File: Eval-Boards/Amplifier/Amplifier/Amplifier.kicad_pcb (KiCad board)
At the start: 2 copper layers, 8 parts

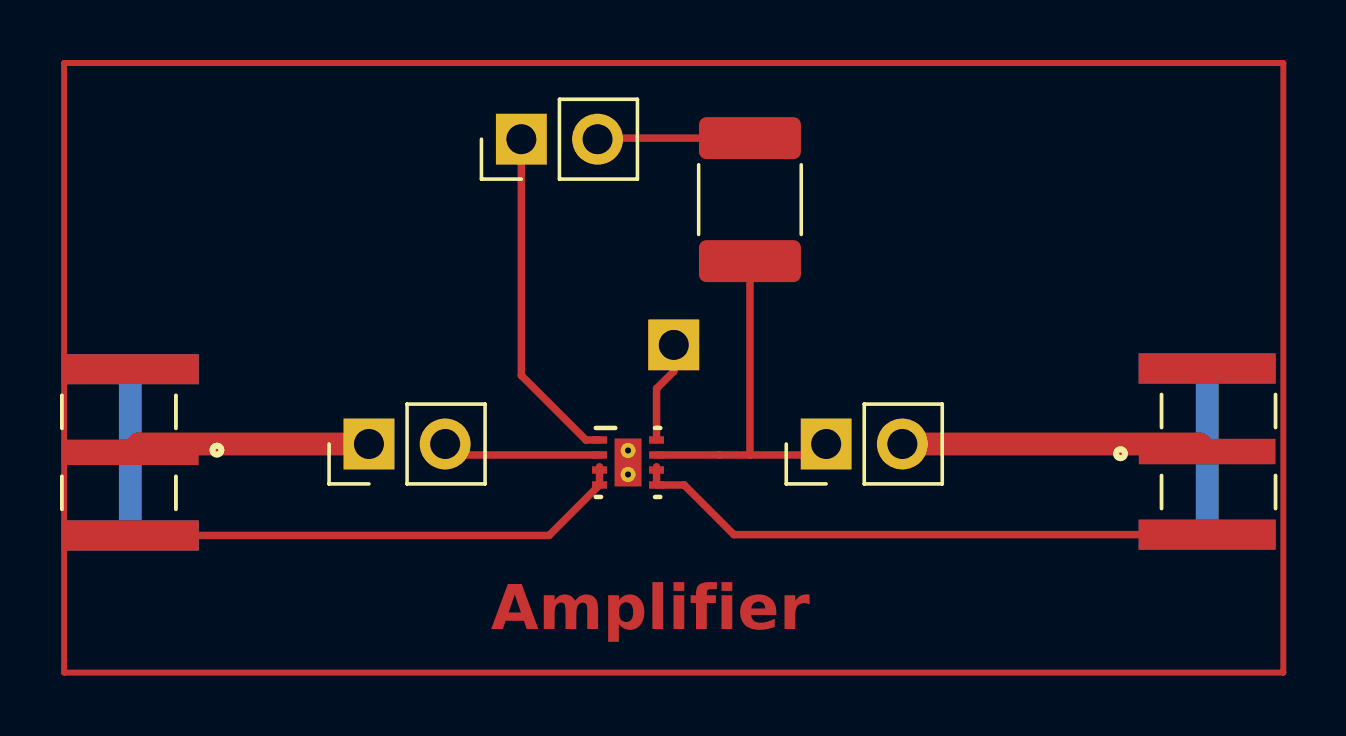
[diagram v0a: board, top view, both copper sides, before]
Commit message: Alot of stuff. Eval board for amp and VCO test
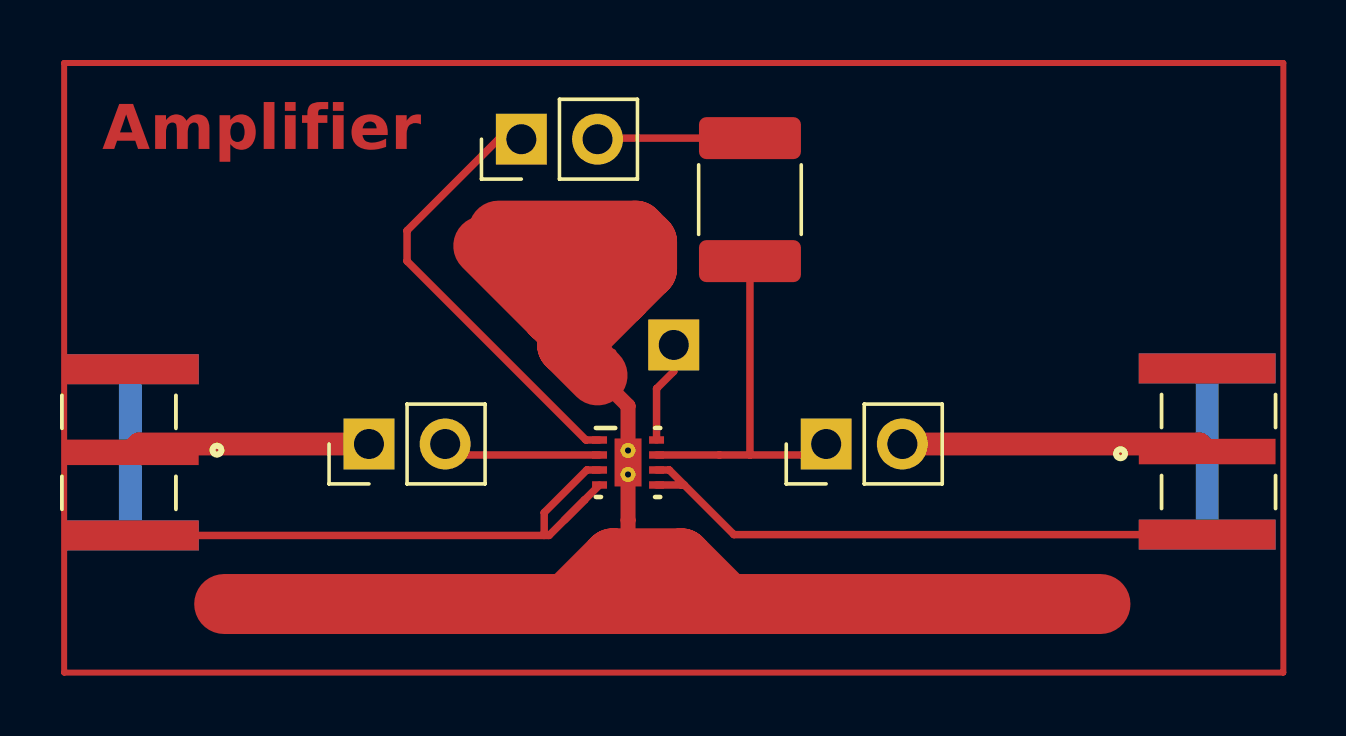
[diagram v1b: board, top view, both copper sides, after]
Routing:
- net (no net): track 103.5 -> 179.9 mm
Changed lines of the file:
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@@
   (gr_rect (start 40.64 35.56) (end 81.28 55.88)
     (stroke (width 0.2) (type default)) (fill none) (layer "F.Cu"))
-  (gr_text "Amplifier" (at 54.864 54.61) (layer "F.Cu")
+  (gr_text "Amplifier" (at 41.91 38.608) (layer "F.Cu")
     (effects (font (size 1.5 1.5) (thickness 0.3) bold) (justify left bottom))
   )
   (segment (start 63.5 48.625999) (end 65.674001 48.625999) (width 0.25) (layer "F.Cu") (net 0))
   (segment (start 53.705999 48.625999) (end 53.34 48.26) (width 0.25) (layer "F.Cu") (net 0))
+  (segment (start 75.184 53.594) (end 57.404 53.594) (width 2) (layer "F.Cu") (net 0))
   (segment (start 43.123001 48.26) (end 42.845001 48.538) (width 0.762) (layer "F.Cu") (net 0))
+  (segment (start 60.810001 49.126001) (end 61.309999 49.625999) (width 0.25) (layer "F.Cu") (net 0))
+  (segment (start 57.311998 50.8) (end 57.992999 50.118999) (width 0.25) (layer "F.Cu") (net 0))
+  (segment (start 61.214 49.625999) (end 61.309999 49.625999) (width 0.25) (layer "F.Cu") (net 0))
+  (segment (start 54.61 41.656) (end 56.896 43.942) (width 2) (layer "F.Cu") (net 0))
+  (segment (start 60.386001 49.625999) (end 61.214 49.625999) (width 0.25) (layer "F.Cu") (net 0))
+  (segment (start 61.214 53.594) (end 61.468 53.594) (width 0.25) (layer "F.Cu") (net 0))
+  (segment (start 58.485999 48.126) (end 58.032 48.126) (width 0.25) (layer "F.Cu") (net 0))
   (segment (start 50.8 48.26) (end 43.123001 48.26) (width 0.762) (layer "F.Cu") (net 0))
-  (segment (start 60.386001 49.625999) (end 61.309999 49.625999) (width 0.25) (layer "F.Cu") (net 0))
+  (segment (start 60.386001 49.126001) (end 60.810001 49.126001) (width 0.25) (layer "F.Cu") (net 0))
+  (segment (start 57.404 44.45) (end 57.404 44.958) (width 2) (layer "F.Cu") (net 0))
+  (segment (start 58.42 45.974) (end 58.166 45.72) (width 0.25) (layer "F.Cu") (net 0))
+  (segment (start 58.485999 49.126001) (end 58.061999 49.126001) (width 0.25) (layer "F.Cu") (net 0))
+  (segment (start 58.039 44.45) (end 57.404 44.45) (width 2) (layer "F.Cu") (net 0))
   (segment (start 60.386001 48.625999) (end 62.484 48.625999) (width 0.25) (layer "F.Cu") (net 0))
+  (segment (start 58.928 46.482) (end 58.928 45.212) (width 0.25) (layer "F.Cu") (net 0))
+  (segment (start 58.032 48.126) (end 52.07 42.164) (width 0.25) (layer "F.Cu") (net 0))
+  (segment (start 57.404 53.594) (end 58.928 52.07) (width 2) (layer "F.Cu") (net 0))
   (segment (start 60.386001 46.416001) (end 60.96 45.842002) (width 0.25) (layer "F.Cu") (net 0))
   (segment (start 65.674001 48.625999) (end 66.04 48.26) (width 0.25) (layer "F.Cu") (net 0))
@@
   (segment (start 78.625251 48.625999) (end 78.74 48.51125) (width 0.25) (layer "F.Cu") (net 0))
   (segment (start 56.803998 51.308) (end 42.845001 51.308) (width 0.25) (layer "F.Cu") (net 0))
+  (segment (start 57.404 53.594) (end 45.974 53.594) (width 2) (layer "F.Cu") (net 0))
   (segment (start 68.58 48.26) (end 78.48875 48.26) (width 0.762) (layer "F.Cu") (net 0))
+  (segment (start 56.896 43.942) (end 57.404 44.45) (width 2) (layer "F.Cu") (net 0))
+  (segment (start 56.642 42.164) (end 58.039 42.164) (width 2) (layer "F.Cu") (net 0))
+  (segment (start 52.07 41.148) (end 55.118 38.1) (width 0.25) (layer "F.Cu") (net 0))
+  (segment (start 52.07 42.164) (end 52.07 41.148) (width 0.25) (layer "F.Cu") (net 0))
+  (segment (start 58.061999 49.126001) (end 56.642 50.546) (width 0.25) (layer "F.Cu") (net 0))
+  (segment (start 58.928 46.482) (end 58.674 46.228) (width 0.25) (layer "F.Cu") (net 0))
+  (segment (start 58.928 52.07) (end 61.214 52.07) (width 2) (layer "F.Cu") (net 0))
   (segment (start 60.386001 48.126) (end 60.386001 46.416001) (width 0.25) (layer "F.Cu") (net 0))
-  (segment (start 56.803998 51.308) (end 58.485999 49.625999) (width 0.25) (layer "F.Cu") (net 0))
+  (segment (start 59.69 41.148) (end 55.118 41.148) (width 2) (layer "F.Cu") (net 0))
   (segment (start 60.96 45.842002) (end 60.96 44.958) (width 0.25) (layer "F.Cu") (net 0))
-  (segment (start 60.386001 49.517998) (end 60.386001 49.018) (width 0.25) (layer "F.Cu") (net 0))
-  (segment (start 58.485999 48.126) (end 58.032 48.126) (width 0.25) (layer "F.Cu") (net 0))
+  (segment (start 59.436 49.276) (end 59.436 50.8) (width 0.5) (layer "F.Cu") (net 0))
+  (segment (start 56.803998 51.308) (end 57.992999 50.118999) (width 0.25) (layer "F.Cu") (net 0))
+  (segment (start 58.674 46.228) (end 58.42 45.974) (width 0.25) (layer "F.Cu") (net 0))
+  (segment (start 60.071 41.529) (end 59.69 41.148) (width 2) (layer "F.Cu") (net 0))
   (segment (start 62.484 48.625999) (end 63.5 48.625999) (width 0.25) (layer "F.Cu") (net 0))
+  (segment (start 56.896 43.307) (end 56.896 43.942) (width 2) (layer "F.Cu") (net 0))
+  (segment (start 59.436 48.476002) (end 59.436 46.99) (width 0.5) (layer "F.Cu") (net 0))
+  (segment (start 61.214 52.07) (end 62.738 53.594) (width 2) (layer "F.Cu") (net 0))
   (segment (start 61.309999 49.625999) (end 62.96525 51.28125) (width 0.25) (layer "F.Cu") (net 0))
-  (segment (start 58.485999 49.018) (end 58.485999 49.517998) (width 0.25) (layer "F.Cu") (net 0))
+  (segment (start 59.436 51.816) (end 59.69 52.07) (width 0.25) (layer "F.Cu") (net 0))
+  (segment (start 58.039 42.164) (end 59.182 43.307) (width 2) (layer "F.Cu") (net 0))
   (segment (start 63.5 38.064) (end 58.456 38.064) (width 0.25) (layer "F.Cu") (net 0))
-  (segment (start 55.88 45.974) (end 55.88 38.1) (width 0.25) (layer "F.Cu") (net 0))
   (segment (start 42.933 48.625999) (end 42.845001 48.538) (width 0.25) (layer "F.Cu") (net 0))
+  (segment (start 56.642 50.546) (end 56.642 51.308) (width 0.25) (layer "F.Cu") (net 0))
+  (segment (start 59.436 46.99) (end 58.928 46.482) (width 0.5) (layer "F.Cu") (net 0))
+  (segment (start 60.071 42.418) (end 59.182 43.307) (width 2) (layer "F.Cu") (net 0))
+  (segment (start 57.992999 50.118999) (end 58.485999 49.625999) (width 0.25) (layer "F.Cu") (net 0))
+  (segment (start 60.071 42.418) (end 60.071 41.529) (width 2) (layer "F.Cu") (net 0))
+  (segment (start 59.182 43.307) (end 58.039 44.45) (width 2) (layer "F.Cu") (net 0))
   (segment (start 63.5 48.625999) (end 63.5 42.164) (width 0.25) (layer "F.Cu") (net 0))
+  (segment (start 59.436 50.8) (end 59.436 51.816) (width 0.5) (layer "F.Cu") (net 0))
+  (segment (start 58.039 42.164) (end 56.896 43.307) (width 2) (layer "F.Cu") (net 0))
+  (segment (start 62.738 53.594) (end 61.468 53.594) (width 2) (layer "F.Cu") (net 0))
   (segment (start 58.456 38.064) (end 58.42 38.1) (width 0.25) (layer "F.Cu") (net 0))
-  (segment (start 58.032 48.126) (end 55.88 45.974) (width 0.25) (layer "F.Cu") (net 0))
+  (segment (start 55.118 38.1) (end 55.88 38.1) (width 0.25) (layer "F.Cu") (net 0))
+  (segment (start 57.404 44.958) (end 58.42 45.974) (width 2) (layer "F.Cu") (net 0))
   (segment (start 58.485999 48.625999) (end 53.705999 48.625999) (width 0.25) (layer "F.Cu") (net 0))
   (segment (start 78.48875 48.26) (end 78.74 48.51125) (width 0.762) (layer "F.Cu") (net 0))
+  (segment (start 59.436 50.8) (end 59.436 53.848) (width 0.4) (layer "F.Cu") (net 0))
   (segment (start 78.74 45.74125) (end 78.74 51.28125) (width 0.762) (layer "B.Cu") (net 0))
   (segment (start 42.845001 45.768) (end 42.845001 51.308) (width 0.762) (layer "B.Cu") (net 0))
